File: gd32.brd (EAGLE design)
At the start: 55 x 70 mm, 23 parts, among them IC1 GD32F450IKH6, IC2 AMS1117-1.5, J1 LCD, U1 W9825G6KH-5

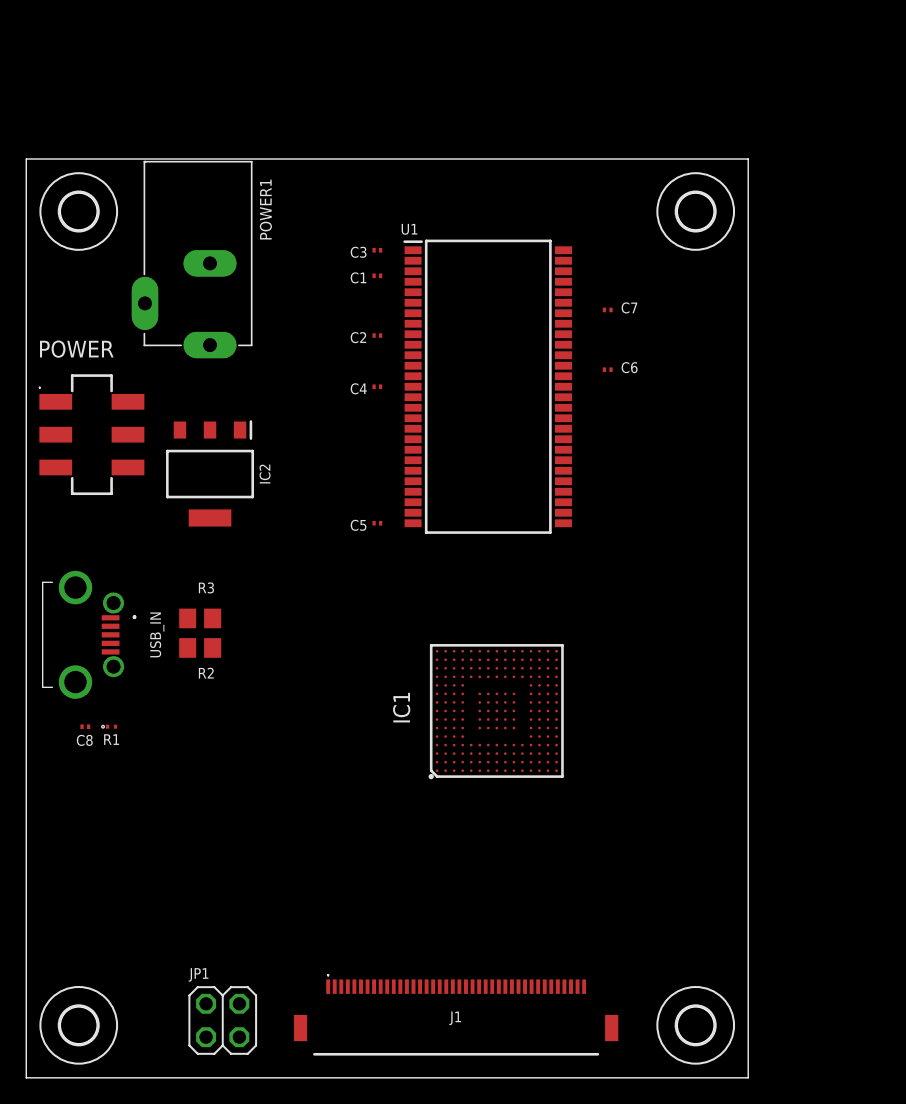
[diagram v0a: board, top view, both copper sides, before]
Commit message: Incremental changes
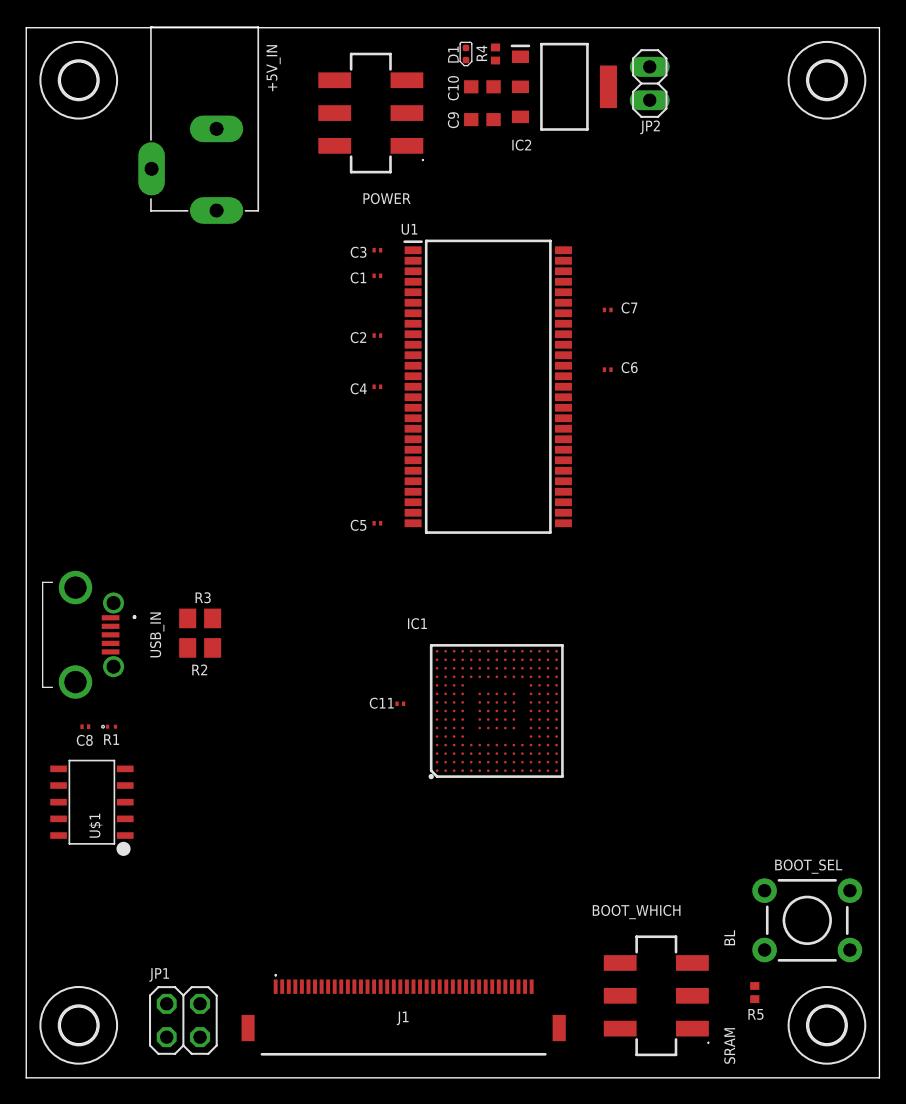
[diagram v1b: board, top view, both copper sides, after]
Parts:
- removed POWER1: DC-005, sjg-power:DCJ3P-14.2X11.0X9.0MM
- added +5V_IN: DC-005, sjg-power:DCJ3P-14.2X11.0X9.0MM
- added BOOT_SEL: B3F-1005, SparkFun:TACTILE-PTH
- added BOOT_WHICH: JS202011SCQN, samacsys:JS202011SCQN
- added C10, C9: 10uF/16v, rcl:C0603
- added C11: 0.1uF, rcl:C0201
- added D1: GRN-0402, Seeed-LED:LED-0402
- added JP2: (no value), pinhead:1X02
- added R4: 470R, rcl:R0402
- added R5: 10K, rcl:R0402
- added U$1: GD32_DEBUG, sjg-stm32:SWD_DEBUG
- IC2: value AMS1117-1.5 -> AMS1117-3.3
- moved IC2 40.0 mm to (41.0, 75.5), turned to 0 degrees
- moved POWER 32.4 mm to (26.2, 73.5), turned to 90 degrees
- moved H4 14.1 mm to (61.0, 76.0)
- moved H1 10.0 mm to (4.00, 76.0)
- moved H3 10.0 mm to (61.0, 4.00)
- moved J1 4.00 mm to (28.8, 4.37)
- moved JP1 3.00 mm to (12.0, 4.37)
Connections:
- new net BOOT0: BOOT_SEL.3, BOOT_SEL.4, IC1.D6, R5.2
- new net N$2: D1.+, R4.2
- new net N$3: C10.1, IC2.2, IC2.4, JP2.2, R4.1
- net +3V3: now also BOOT_SEL.1, BOOT_SEL.2, BOOT_WHICH.1, BOOT_WHICH.6, JP2.1, U$1.P1; no longer IC2.2, IC2.4
- net +5V: now also C9.1
- net GND: now also +5V_IN.-1, +5V_IN.-2, BOOT_WHICH.3, BOOT_WHICH.4, C10.2, C11.2, C9.2, R5.1, U$1.P3, U$1.P5, U$1.P9; no longer POWER1.-1, POWER1.-2
- net PA13: now also U$1.P2
- net PA14: now also U$1.P4
- net PB10: now also U$1.P6
- net PB11: now also U$1.P8
- net PB2: now also BOOT_WHICH.2, BOOT_WHICH.5
- net PB4: now also C11.1, U$1.P10
- net V+: now also +5V_IN.+; no longer POWER1.+
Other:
- board size 55 x 70 mm -> 65 x 80 mm
- board text added: "BL"
- board text added: "SRAM"
